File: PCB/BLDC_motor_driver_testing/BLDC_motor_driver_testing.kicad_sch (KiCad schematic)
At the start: 18 parts, among them J1 PWR, J2 SD_IN, J3 PWM_IN, J4 IN_SENSE_ADC, U1 AMS1117-3.3

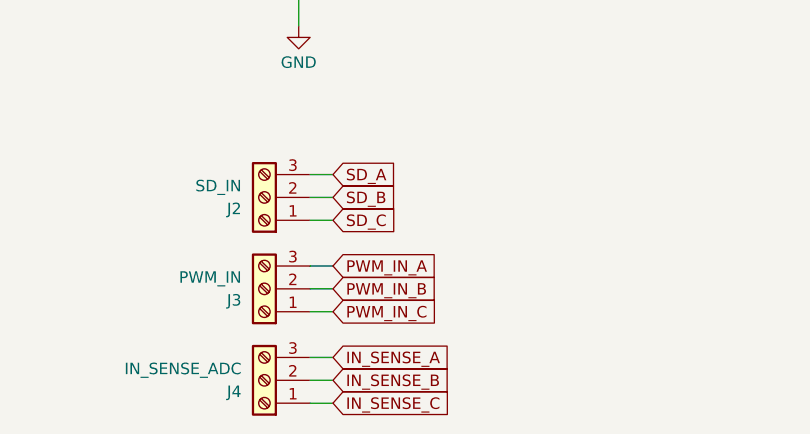
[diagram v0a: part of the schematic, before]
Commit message: Test driver layout...
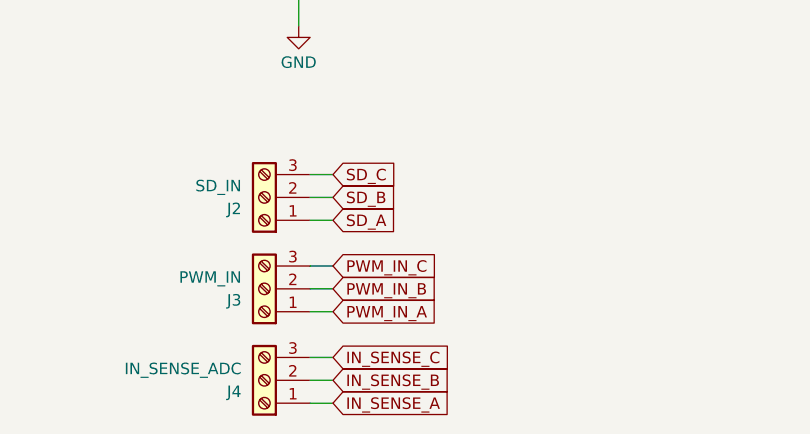
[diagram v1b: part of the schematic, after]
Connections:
- net IN_SENSE_A: now also J4.1 (Pin_1); no longer J4.3 (Pin_3)
- net IN_SENSE_C: now also J4.3 (Pin_3); no longer J4.1 (Pin_1)
- net PWM_IN_A: now also J3.1 (Pin_1); no longer J3.3 (Pin_3)
- net PWM_IN_C: now also J3.3 (Pin_3); no longer J3.1 (Pin_1)
- net SD_A: now also J2.1 (Pin_1); no longer J2.3 (Pin_3)
- net SD_C: now also J2.3 (Pin_3); no longer J2.1 (Pin_1)
